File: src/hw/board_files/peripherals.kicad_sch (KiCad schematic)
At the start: 26 parts, among them J7 Conn_01x04, J8 Molex 104031-0811, Q1 PMOS, U5 NEO-M9N, U6 BQ27427, U7 SHT30-DIS

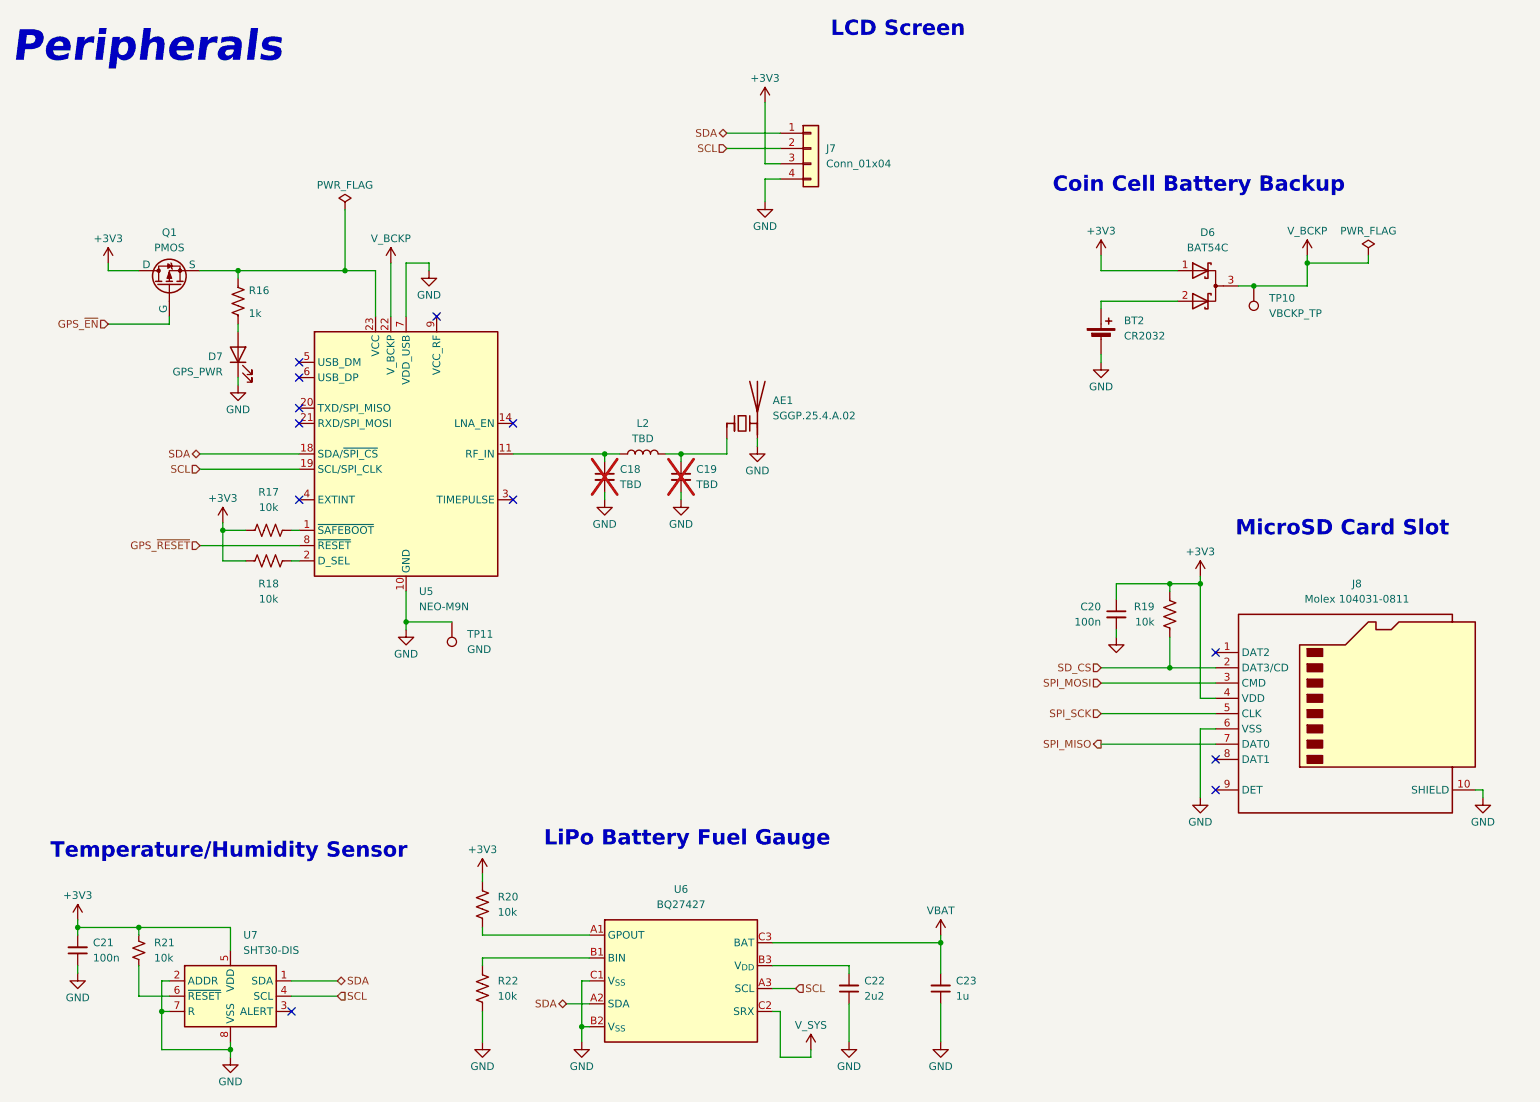
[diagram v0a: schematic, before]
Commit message: Minor schematic updates
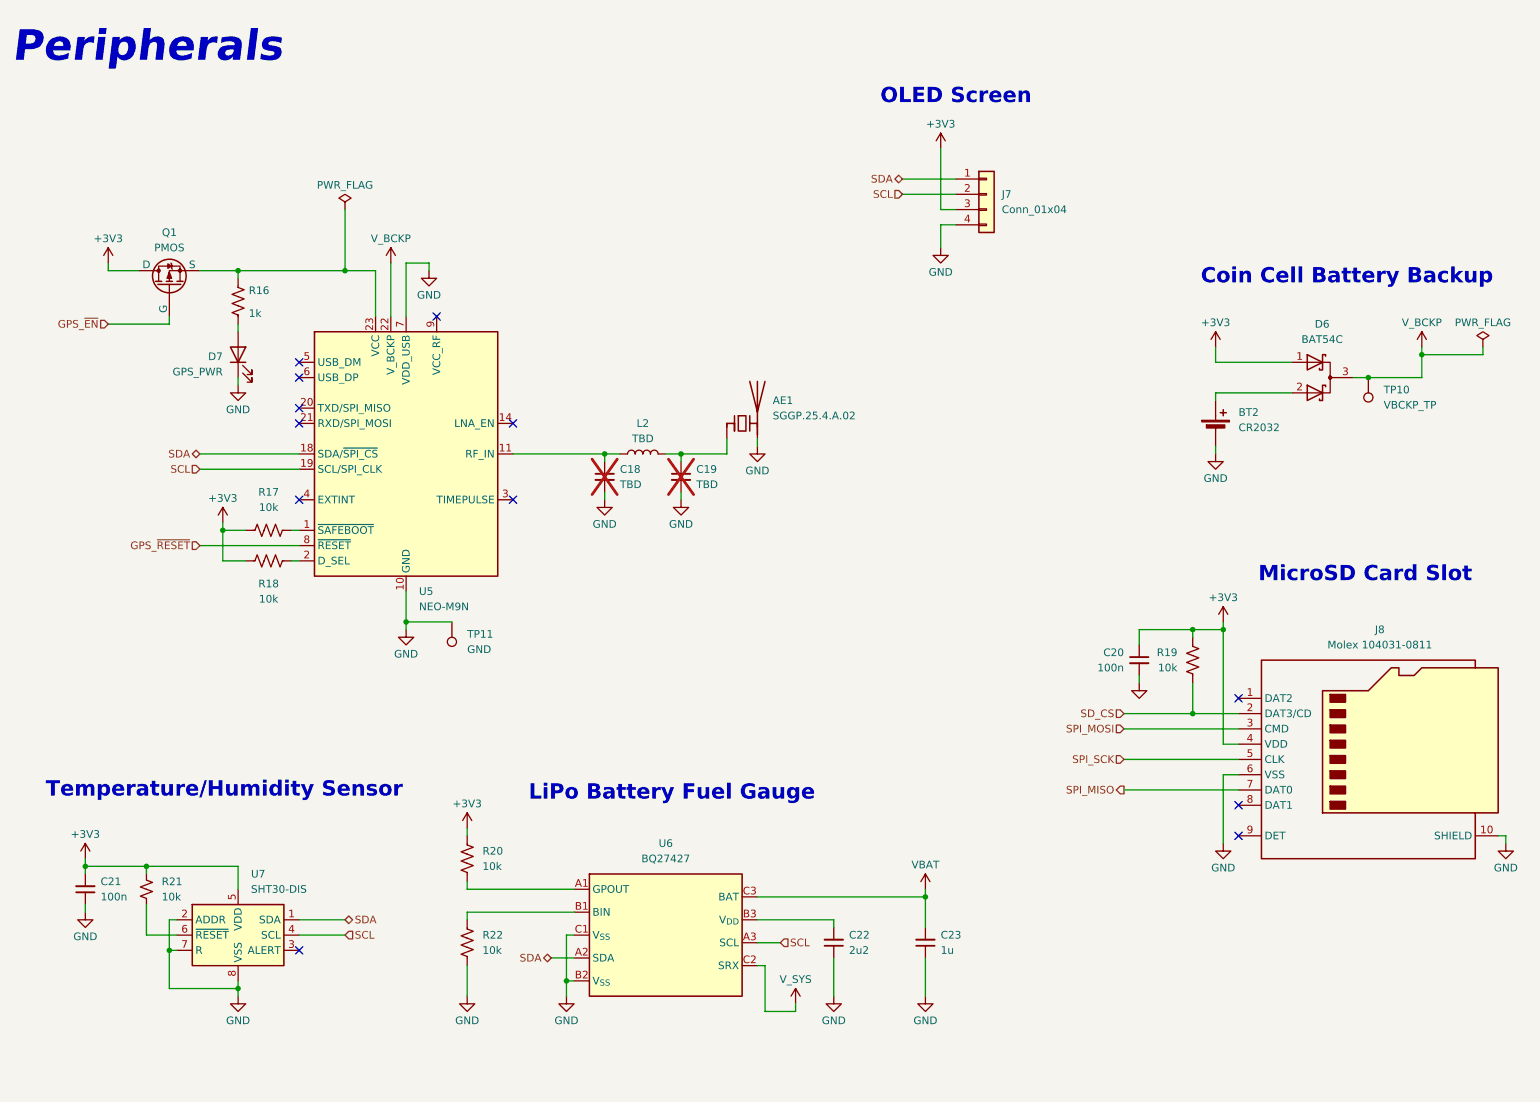
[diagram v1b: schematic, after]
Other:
- note added: "OLED Screen"
- note removed: "LCD Screen"
- moved on the sheet: BT2, C20, C21, C22, C23, D6, J7, J8, R19, R20, R21, R22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
